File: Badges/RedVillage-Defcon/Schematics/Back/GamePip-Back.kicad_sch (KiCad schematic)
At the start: 44 parts, among them J1 2.8" Display, J2 USB_C_Plug_USB2.0, J3 Conn_01x03, Q1 Q_PMOS_DGS, Q2 Q_NPN_BCE, SW1 Up, SW2 Down, SW3 Left, SW4 A, SW5 Right, SW6 B, SW7 Start, SW8 Select, SW9 RotaryEncoder_Switch, U1 XDS_TX4310B

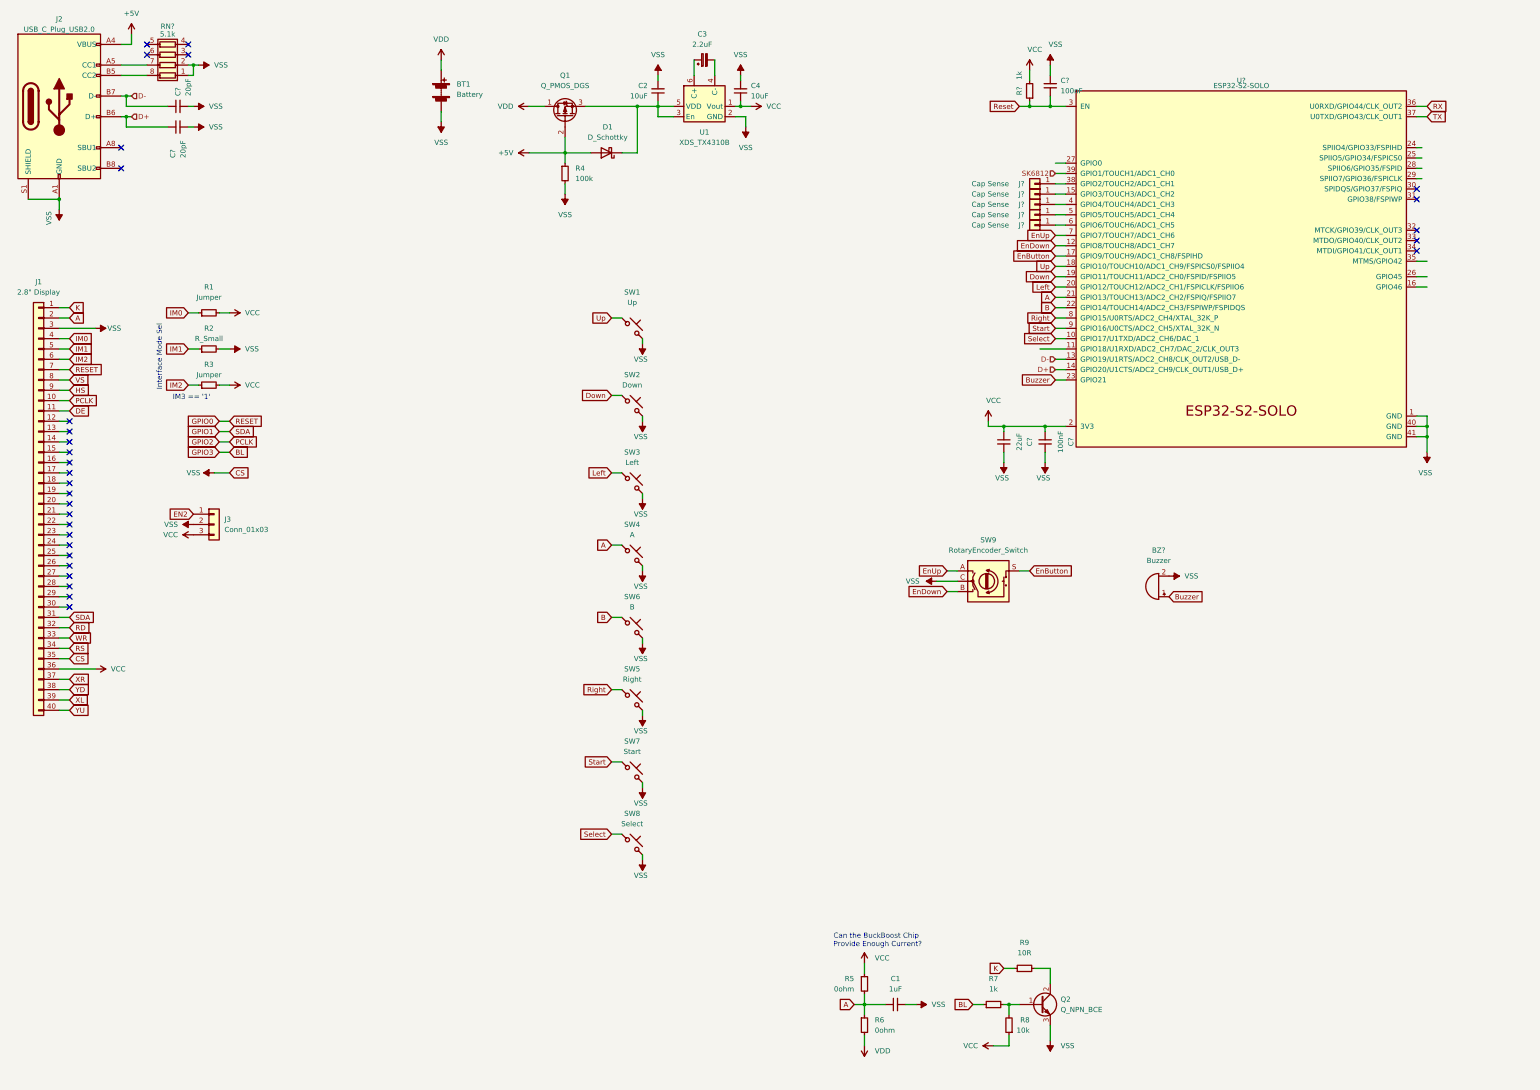
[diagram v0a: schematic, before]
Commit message: update
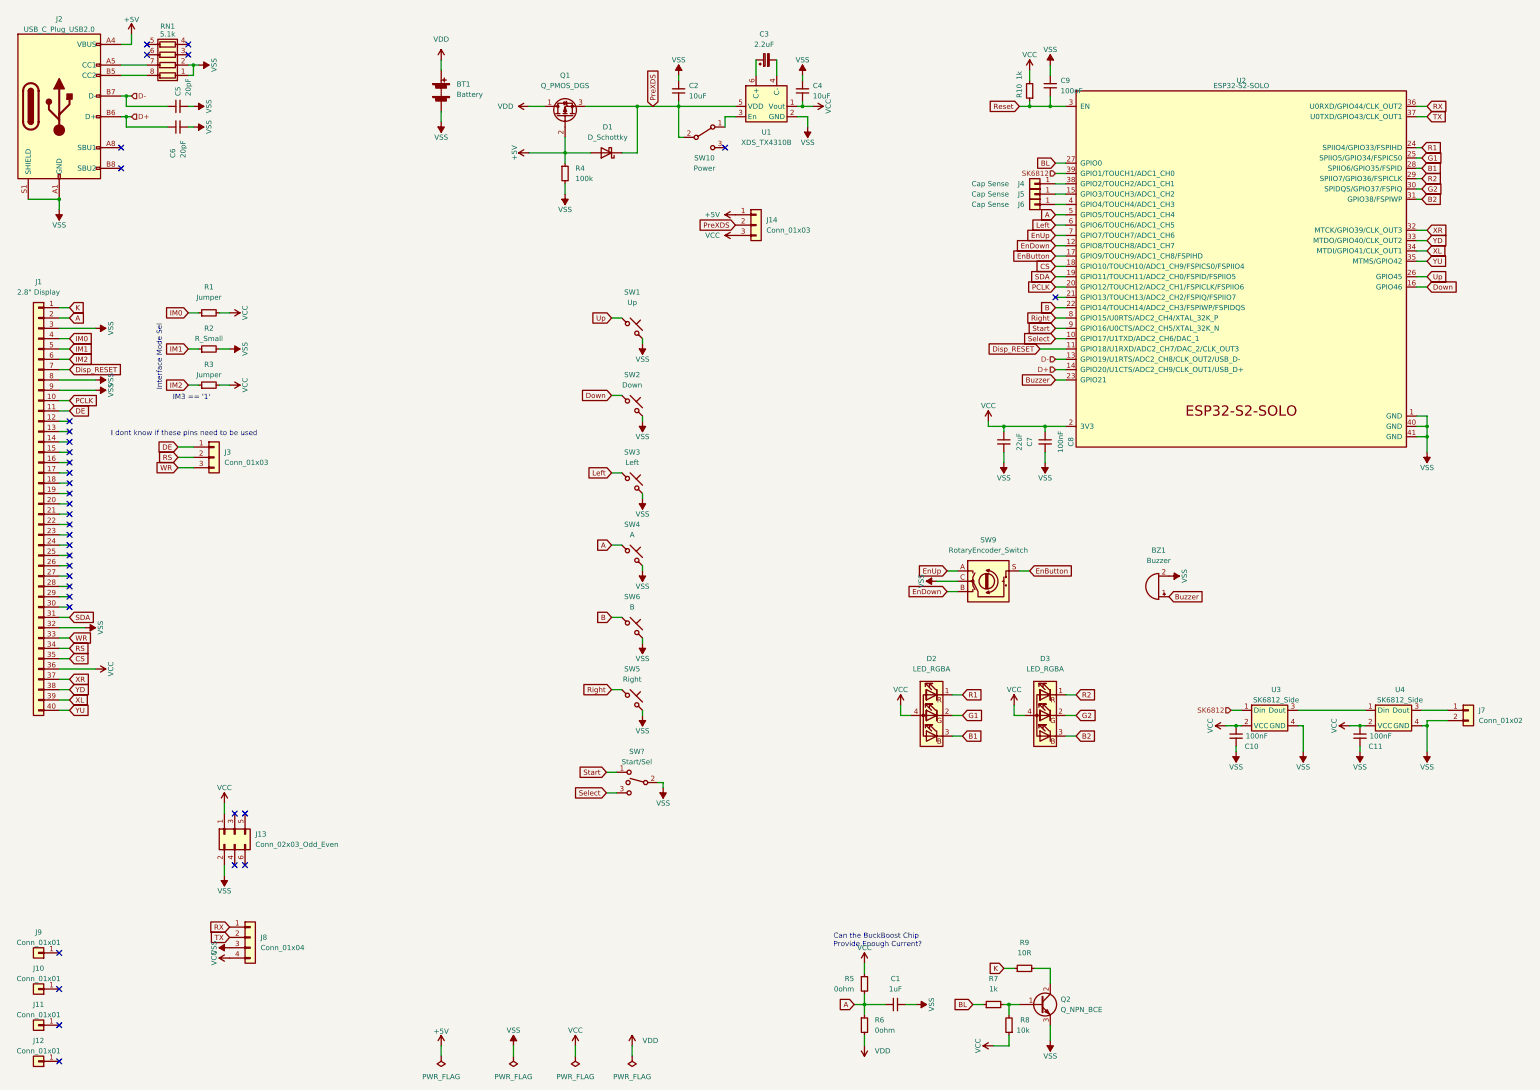
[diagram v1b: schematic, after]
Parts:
- removed J? (x2): Cap Sense, Bsides22:CapSense, symbol Connector_Generic:Conn_01x01
- removed SW7: Start, symbol Switch:SW_Push_45deg
- removed SW8: Select, symbol Switch:SW_Push_45deg
- added C10, C11: 100nF, Capacitor_SMD:C_0805_2012Metric, symbol Device:C_Small
- added D2, D3: LED_RGBA, RedVillage:XL-3227RGB_LED, symbol Device:LED_RGBA
- added J10, J11, J12, J9: Conn_01x01, cafebabe:SMD Spacer M2.5, symbol Connector_Generic:Conn_01x01
- added J13: Conn_02x03_Odd_Even, Connector_PinSocket_2.54mm:PinSocket_2x03_P2.54mm_Vertical, symbol Connector_Generic:Conn_02x03_Odd_Even
- added J14: Conn_01x03, Connector_PinSocket_2.54mm:PinSocket_1x03_P2.54mm_Vertical, symbol Connector_Generic:Conn_01x03
- added J7: Conn_01x02, Connector_PinSocket_2.54mm:PinSocket_1x02_P2.54mm_Vertical, symbol Connector_Generic:Conn_01x02
- added J8: Conn_01x04, Connector_PinSocket_2.54mm:PinSocket_1x04_P2.54mm_Vertical, symbol Connector_Generic:Conn_01x04
- added SW10: Power, UE-ButtonSwitch:SK-3296S_switch, symbol Switch:SW_SPDT
- added SW?: Start/Sel, symbol Switch:SW_SPDT_MSM
- added U3, U4: SK6812_Side, Bsides22:SK6812_Side, symbol BSides22:SK6812_Side
- C1, C3: footprint (none) -> Capacitor_SMD:C_0805_2012Metric
- D1: footprint (none) -> Diode_SMD:D_SOD-123
- R1, R2, R3, R4, R5, R6, R7, R8, R9: footprint (none) -> Resistor_SMD:R_0815_2038Metric
- SW1, SW2, SW3, SW4, SW5, SW6: footprint (none) -> RedVillage:BZCN-TSC005A_Button
- SW9: footprint (none) -> RedVillage:SIQ-02FVS3_Encoder
- gave numbers to parts that had none: 12
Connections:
- net EN2 is gone; now on net DE: J3.1 (Pin_1)
- net GPIO0 is gone; now on net Disp_RESET: J1.7 (Pin_7)
- net HS is gone; now on net VSS: J1.9 (Pin_9)
- net RD is gone; now on net VSS: J1.32 (Pin_32)
- net VS is gone; now on net VSS: J1.8 (Pin_8)
- net +5V: now also J14.1 (Pin_1)
- net A: now also U2.5 (GPIO5/TOUCH5/ADC1_CH4); no longer U2.21 (GPIO13/TOUCH13/ADC2_CH2/FSPIQ/FSPIIO7)
- net BL: now also U2.27 (GPIO0)
- net Down: now also U2.16 (GPIO46); no longer U2.19 (GPIO11/TOUCH11/ADC2_CH0/FSPID/FSPIIO5)
- net Left: now also U2.6 (GPIO6/TOUCH6/ADC1_CH5); no longer U2.20 (GPIO12/TOUCH12/ADC2_CH1/FSPICLK/FSPIIO6)
- net RS: now also J3.2 (Pin_2)
- net RX: now also J8.1 (Pin_1)
- net SK6812: now also U3.1 (Din)
- net Select: now also SW?.3
- net Start: now also SW?.1
- net TX: now also J8.2 (Pin_2)
- net Up: now also U2.26 (GPIO45); no longer U2.18 (GPIO10/TOUCH10/ADC1_CH9/FSPICS0/FSPIIO4)
- net VCC: now also C10.1, C11.1, D2.4 (A), D3.4 (A), J13.1 (Pin_1), J14.3 (Pin_3), J8.4 (Pin_4), U3.2 (VCC), U4.2 (VCC); no longer J3.3 (Pin_3)
- net VSS: now also C10.2, C11.2, J13.2 (Pin_2), J7.2 (Pin_2), J8.3 (Pin_3), SW?.2, U3.4 (GND), U4.4 (GND); no longer J1.35 (Pin_35), J3.2 (Pin_2)
- net WR: now also J3.3 (Pin_3)
- net XL: now also U2.34 (MTDI/GPIO41/CLK_OUT1)
- net XR: now also U2.32 (MTCK/GPIO39/CLK_OUT3)
- net YD: now also U2.33 (MTDO/GPIO40/CLK_OUT2)
- net YU: now also U2.35 (MTMS/GPIO42)
- net PreXDS: now reaches C2.1, D1.1 (K), Q1.3 (S), U1.5 (VDD)
- net PreXDS: now also J14.2 (Pin_2), SW10.2 (B); no longer U1.3 (En)
- net Disp_RESET: now reaches U2.11 (GPIO18/U1RXD/ADC2_CH7/DAC_2/CLK_OUT3)
- net R1: now reaches U2.24 (SPIIO4/GPIO33/FSPIHD)
- net R1: now also D2.1 (RK)
- net G1: now reaches U2.25 (SPIIO5/GPIO34/FSPICS0)
- net G1: now also D2.2 (GK)
- net B1: now reaches U2.28 (SPIIO6/GPIO35/FSPID)
- net B1: now also D2.3 (BK)
- net R2: now reaches U2.29 (SPIIO7/GPIO36/FSPICLK)
- net R2: now also D3.1 (RK)
- net G2: now reaches U2.30 (SPIDQS/GPIO37/FSPIQ)
- net G2: now also D3.2 (GK)
- net B2: now reaches U2.31 (GPIO38/FSPIWP)
- net B2: now also D3.3 (BK)
- net GPIO1 renamed SDA
- net SDA: now also U2.19 (GPIO11/TOUCH11/ADC2_CH0/FSPID/FSPIIO5)
- net GPIO2 renamed PCLK
- net PCLK: now also U2.20 (GPIO12/TOUCH12/ADC2_CH1/FSPICLK/FSPIIO6)
- new net: U3.3 (Dout), U4.1 (Din)
- new net: J7.1 (Pin_1), U4.3 (Dout)
- new net: SW10.1 (A), U1.3 (En)
- new net CS: J1.35 (Pin_35), U2.18 (GPIO10/TOUCH10/ADC1_CH9/FSPICS0/FSPIIO4)
- no-connect marks 30 -> 35
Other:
- note added: "I dont know if these pins need to be used"
- moved on the sheet: C2, C3, C4, U1

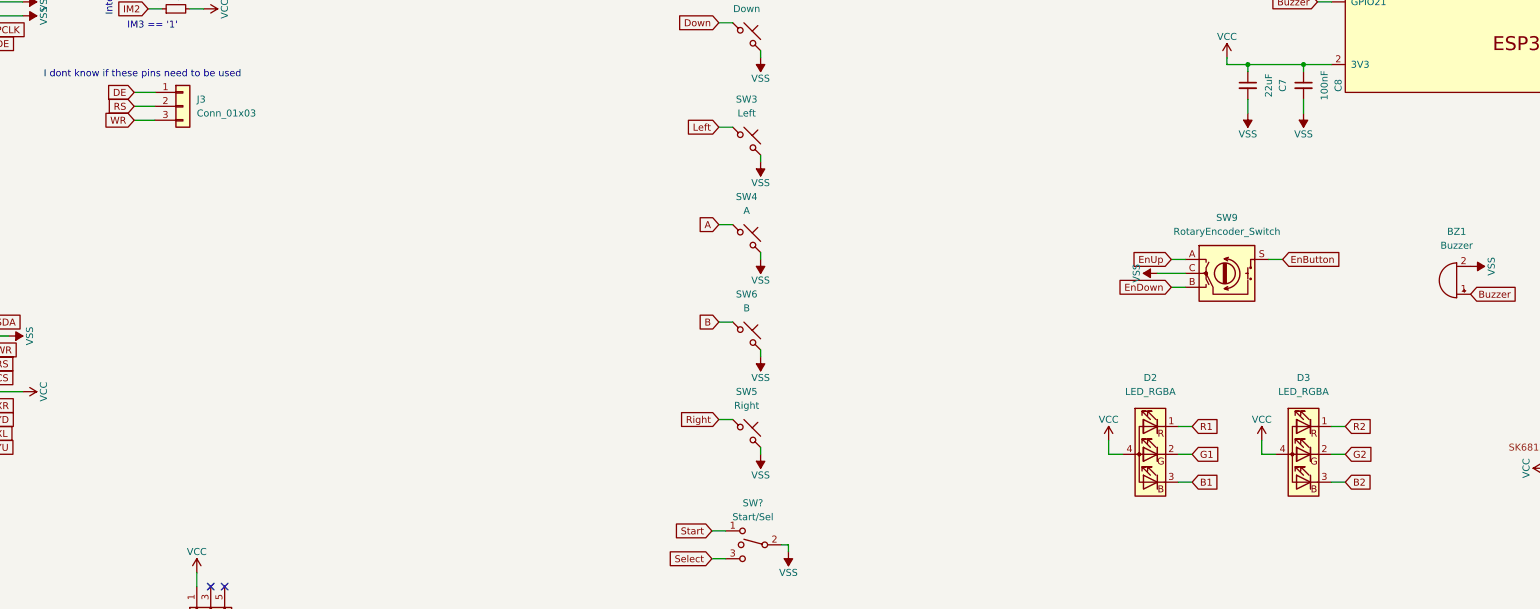
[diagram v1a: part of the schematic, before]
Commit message: Further updates
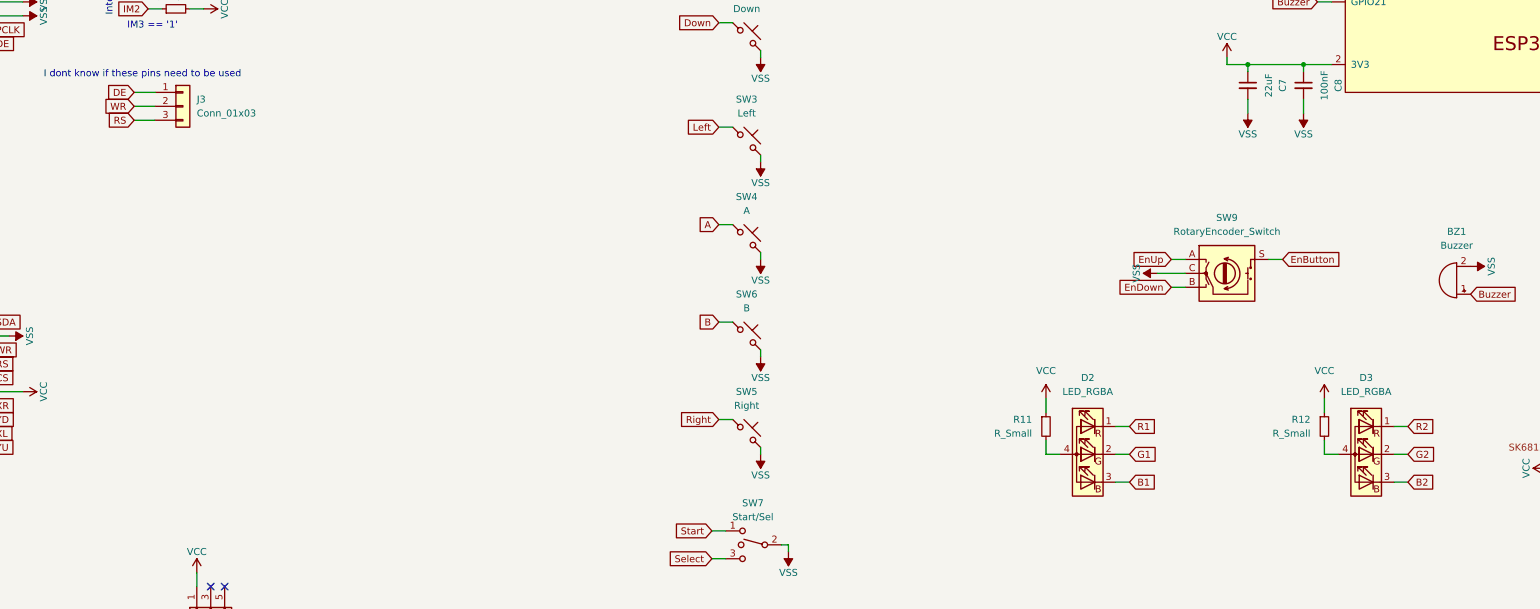
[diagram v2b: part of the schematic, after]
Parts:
- added R11, R12: R_Small, Resistor_SMD:R_0805_2012Metric, symbol Device:R_Small
- BT1: footprint (none) -> RedVillage:AA_TH
- C3: footprint Capacitor_SMD:C_0805_2012Metric -> RedVillage:C_0805_2012Metric
- J1: footprint (none) -> RedVillage:Omron_XF2M-4015-1A_1x40-1MP_P0.5mm_Horizontal
- Q1, Q2: footprint (none) -> Package_TO_SOT_SMD:SOT-23
- R1, R2, R3, R4, R5, R6, R7, R8, R9: footprint Resistor_SMD:R_0815_2038Metric -> Resistor_SMD:R_0805_2012Metric
- SW7: renamed from SW?; footprint (none) -> RedVillage:StartSel
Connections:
- net RS: now also J3.3 (Pin_3); no longer J3.2 (Pin_2)
- net VCC: now also R11.1, R12.1; no longer D2.4 (A), D3.4 (A)
- net WR: now also J3.2 (Pin_2); no longer J3.3 (Pin_3)
- new net: D3.4 (A), R12.2
- new net: D2.4 (A), R11.2
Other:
- moved on the sheet: D2, D3
